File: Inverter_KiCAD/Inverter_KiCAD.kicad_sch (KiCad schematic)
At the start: 12 parts, among them J101 Conn_02x19_Odd_Even, J103 Conn_02x19_Odd_Even, J2 Conn_01x03, J901 Conn_01x02

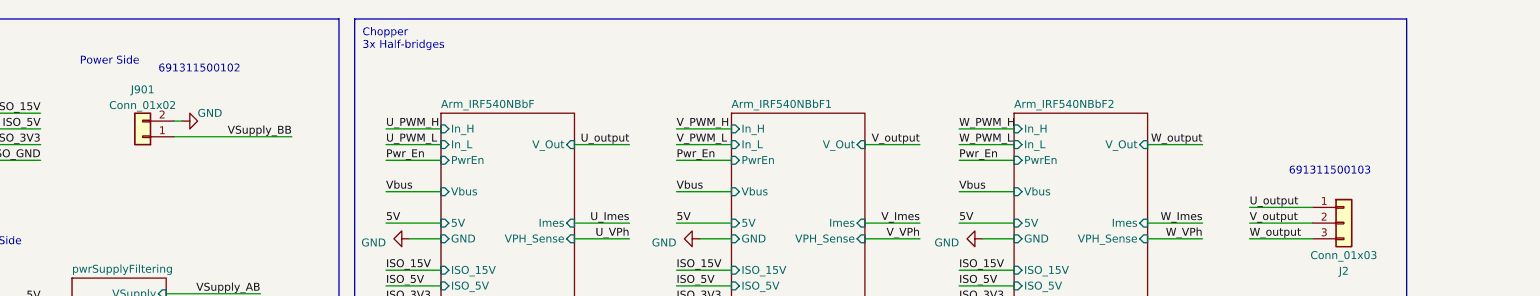
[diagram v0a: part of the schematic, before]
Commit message: Update KiCAD
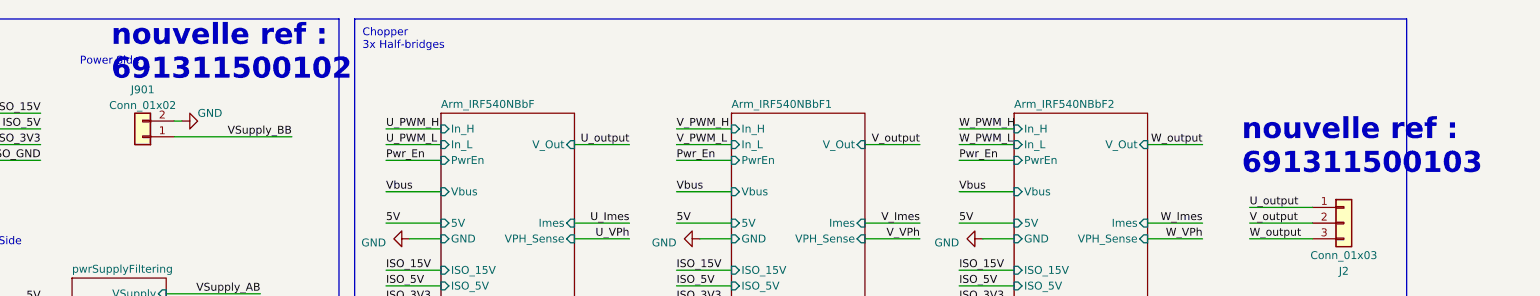
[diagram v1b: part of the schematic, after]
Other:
- note added: "nouvelle ref : 691311500102"
- note added: "nouvelle ref : 691311500103"
- note removed: "691311500102"
- note removed: "691311500103"
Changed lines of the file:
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@@
     (effects (font (size 1.27 1.27)) (justify left bottom))
   )
-  (text "691311500103" (at 264.16 39.37 0)
-    (effects (font (size 1.27 1.27)) (justify left bottom))
+  (text "nouvelle ref : \n691311500103" (at 256.54 39.37 0)
+    (effects (font (size 3.4 3.4) (thickness 0.762) bold) (justify left bottom))
   )
   (text "PA8" (at 92.71 125.73 0)
@@
     (effects (font (size 1.27 1.27)) (justify left bottom))
   )
-  (text "691311500102" (at 81.28 22.86 0)
-    (effects (font (size 1.27 1.27)) (justify left bottom))
+  (text "nouvelle ref : \n691311500102" (at 73.66 24.13 0)
+    (effects (font (size 3.4 3.4) (thickness 0.68) bold) (justify left bottom))
   )
   (text "E5V" (at 52.07 102.87 0)
